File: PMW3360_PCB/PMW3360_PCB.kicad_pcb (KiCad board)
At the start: 2 copper layers, 26.4 x 35.2 mm, 19 parts, among them J1 Conn_01x08, U1 PMW3360DM-T2QU, U2 TPS73601DBV

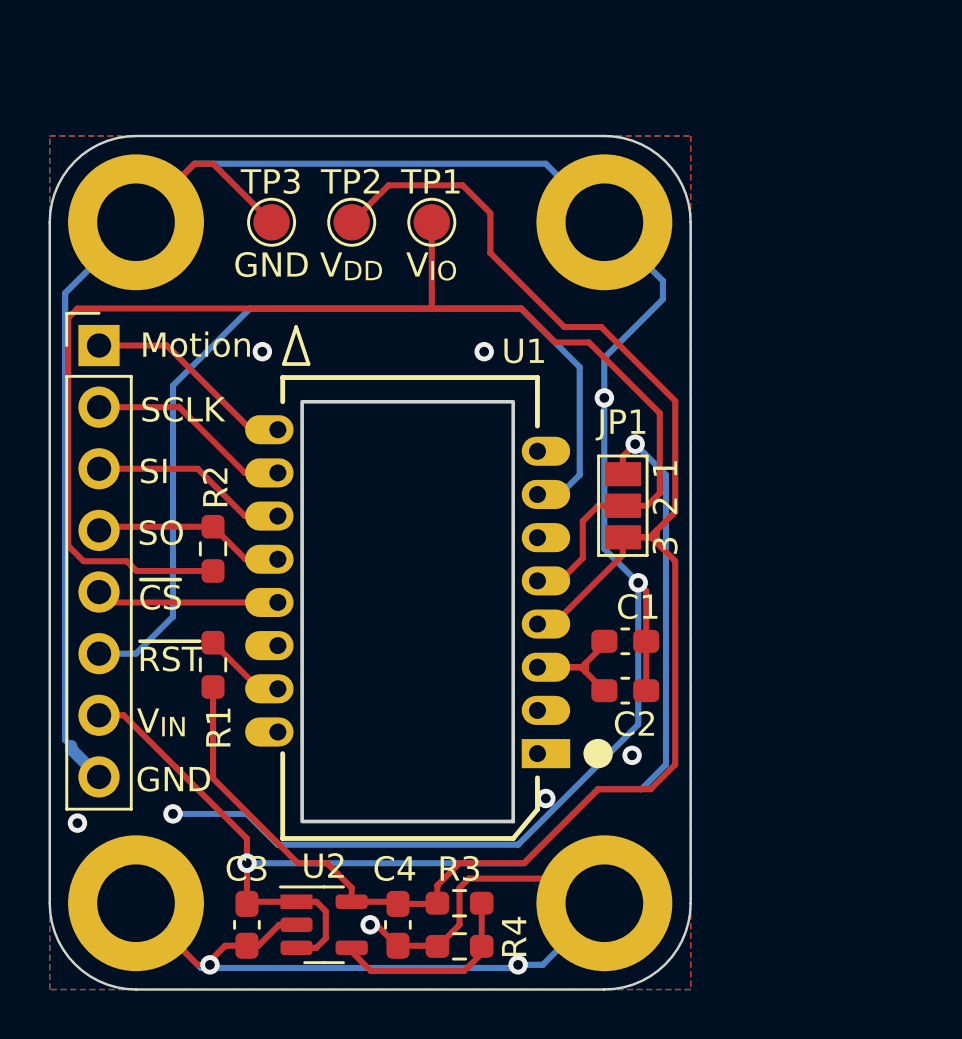
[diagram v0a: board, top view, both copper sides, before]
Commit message: Update 2.1
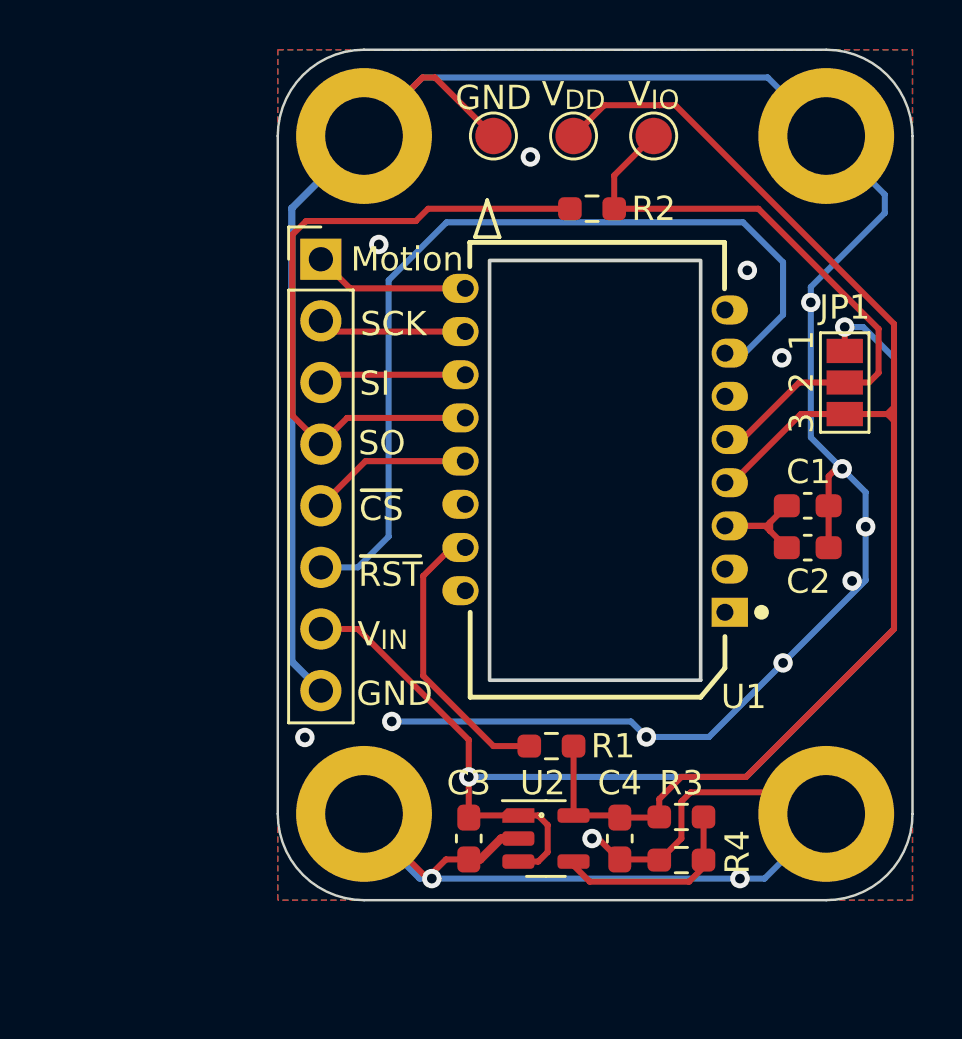
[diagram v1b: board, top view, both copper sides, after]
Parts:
- R3: value 28k -> Adj_R1
- R4: value 56.2k -> Adj_R2
- U1: footprint PMW3360_PCB:16pin‐DIP(PMW3360DM-T2QU) -> PMW3360_PCB:PMW3360DM-T2QU 16Pin
- moved R2 21.0 mm to (236.1, 124.6), turned to 180 degrees
- moved R1 14.3 mm to (234.4, 146.7), turned to 180 degrees
- moved U1 12.2 mm to (236.2, 135.1)
- moved JP1 10.5 mm to (246.5, 131.7)
- moved REF** 10.1 mm to (226.7, 149.5)
- moved REF** 10.0 mm to (226.7, 121.6)
- moved REF** 9.86 mm to (245.7, 149.5)
- moved R3 9.81 mm to (239.8, 149.7)
- moved R4 9.81 mm to (239.8, 151.4)
- moved TP1 9.81 mm to (238.6, 121.6)
- moved TP3 9.81 mm to (232.0, 121.6)
- moved C3 9.81 mm to (231.0, 150.5)
- moved J1 9.81 mm to (224.9, 126.7)
- moved U2 9.81 mm to (234.2, 150.5)
- moved TP2 9.81 mm to (235.3, 121.6)
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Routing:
- net V_IO: track 56.7 -> 25.7 mm
- net /MISO: track 7.74 -> 27.3 mm
- net VDD: track 71.0 -> 58.5 mm
- net Net-(R1-Pad2): track 3.46 -> 11.5 mm
- net GND: track 145.4 -> 142.7 mm, vias 11 -> 15
- net /MOTION: track 8.56 -> 6.55 mm
- net /SCLK: track 8.24 -> 6.23 mm
- net /RESET: track 38.8 -> 36.9 mm
- net /MOSI: track 7.93 -> 6.18 mm
- net V_IN: track 51.0 -> 51.9 mm
- net Net-(C1-Pad1): track 6.81 -> 6.17 mm
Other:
- board size 26.4 x 35.2 mm -> 26.2 x 35.1 mm
- board text added: "PMW3360 PCB Rev 2.1"
- board text added: "SCK"
- board text removed: "PMW3360 PCB Rev 2.0"
- board text removed: "SCLK"
